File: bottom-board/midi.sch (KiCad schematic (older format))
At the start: 14 parts, among them P6 AudioJack3, P7 AudioJack3, Q12 2N7002, Q13 2N7002, U11 6N137S

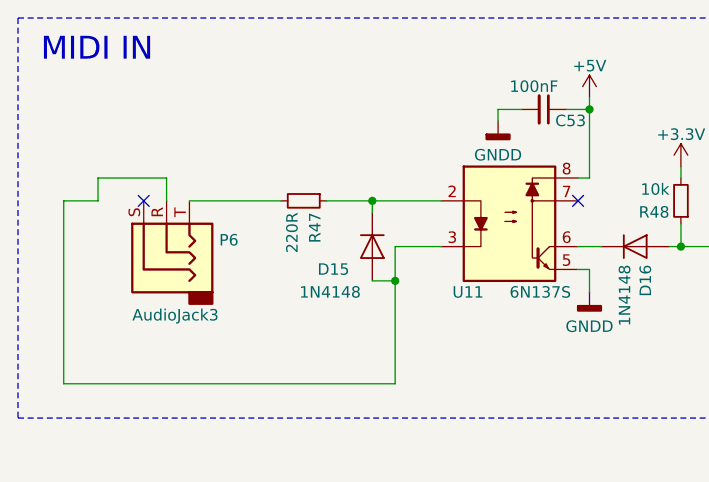
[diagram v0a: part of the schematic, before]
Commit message: add fabrication files bottom board
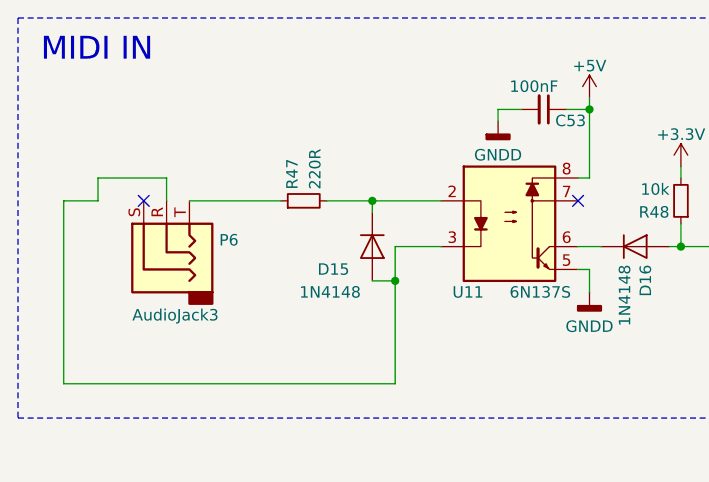
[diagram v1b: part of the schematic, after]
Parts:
- P6, P7: MPN (none) -> SJ-3523-SMT-TR
- R47: footprint Resistor_SMD:R_0805_2012Metric -> Resistor_SMD:R_0603_1608Metric; MPN ERJ-P06J221V -> RL73N1JR22JTD
- R49, R50: MPN ERJ-P06J221V -> RL73N1JR22JTD
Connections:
- net at D15.1 (K), U11.2: now also R47.2; no longer R47.1
- net at P6.T: now also R47.1; no longer R47.2
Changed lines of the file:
@@
 $EndDescr
-$Comp
-L bottom-board-rescue:R_Small R47
-U 1 1 550EB368
-P 2850 3550
-F 0 "R47" H 2900 3600 50  0000 L CNN
-F 1 "220R" H 2900 3500 50  0000 L CNN
-F 2 "Resistor_SMD:R_0805_2012Metric" H 2850 3550 60  0001 C CNN
-F 3 "" H 2850 3550 60  0000 C CNN
-F 4 "ERJ-P06J221V" H 100 0   50  0001 C CNN "MPN"
-	1    2850 3550
-	0    1    1    0
-$EndComp
 $Comp
 L bottom-board-rescue:R_Small R49
@@
 F 2 "Resistor_SMD:R_0603_1608Metric" H 6500 3350 60  0001 C CNN
 F 3 "" H 6500 3350 60  0000 C CNN
-F 4 "ERJ-P06J221V" H 200 0   50  0001 C CNN "MPN"
+F 4 "RL73N1JR22JTD" H 200 0   50  0001 C CNN "MPN"
 	1    6500 3350
 	-1   0    0    1
@@
 F 2 "Resistor_SMD:R_0603_1608Metric" H 7700 3550 60  0001 C CNN
 F 3 "" H 7700 3550 60  0000 C CNN
-F 4 "ERJ-P06J221V" H 350 0   50  0001 C CNN "MPN"
+F 4 "RL73N1JR22JTD" H 350 0   50  0001 C CNN "MPN"
 	1    7700 3550
 	0    -1   -1   0
@@
 F 2 "Connector_Audio:Jack_3.5mm_CUI_SJ-3523-SMT_Horizontal" H 7050 3750 50  0001 C CNN
 F 3 "~" H 7050 3750 50  0001 C CNN
+F 4 "SJ-3523-SMT-TR" V 7050 3750 50  0001 C CNN "MPN"
 	1    7050 3750
 	0    -1   -1   0
@@
 F 2 "Connector_Audio:Jack_3.5mm_CUI_SJ-3523-SMT_Horizontal" H 2250 3750 50  0001 C CNN
 F 3 "~" H 2250 3750 50  0001 C CNN
+F 4 "SJ-3523-SMT-TR" V 2250 3750 50  0001 C CNN "MPN"
 	1    2250 3750
 	0    -1   -1   0
@@
 Wire Wire Line
 	4150 3750 4050 3750
+$Comp
+L bottom-board-rescue:R_Small R47
+U 1 1 5DFAB84B
+P 2850 3550
+F 0 "R47" H 2900 3600 50  0000 L CNN
+F 1 "220R" H 2900 3500 50  0000 L CNN
+F 2 "Resistor_SMD:R_0603_1608Metric" H 2850 3550 60  0001 C CNN
+F 3 "" H 2850 3550 60  0000 C CNN
+F 4 "RL73N1JR22JTD" H -3450 200 50  0001 C CNN "MPN"
+	1    2850 3550
+	0    -1   -1   0
+$EndComp
 $EndSCHEMATC
